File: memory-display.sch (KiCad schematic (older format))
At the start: 1 part, among them J1 TEENSY-LC

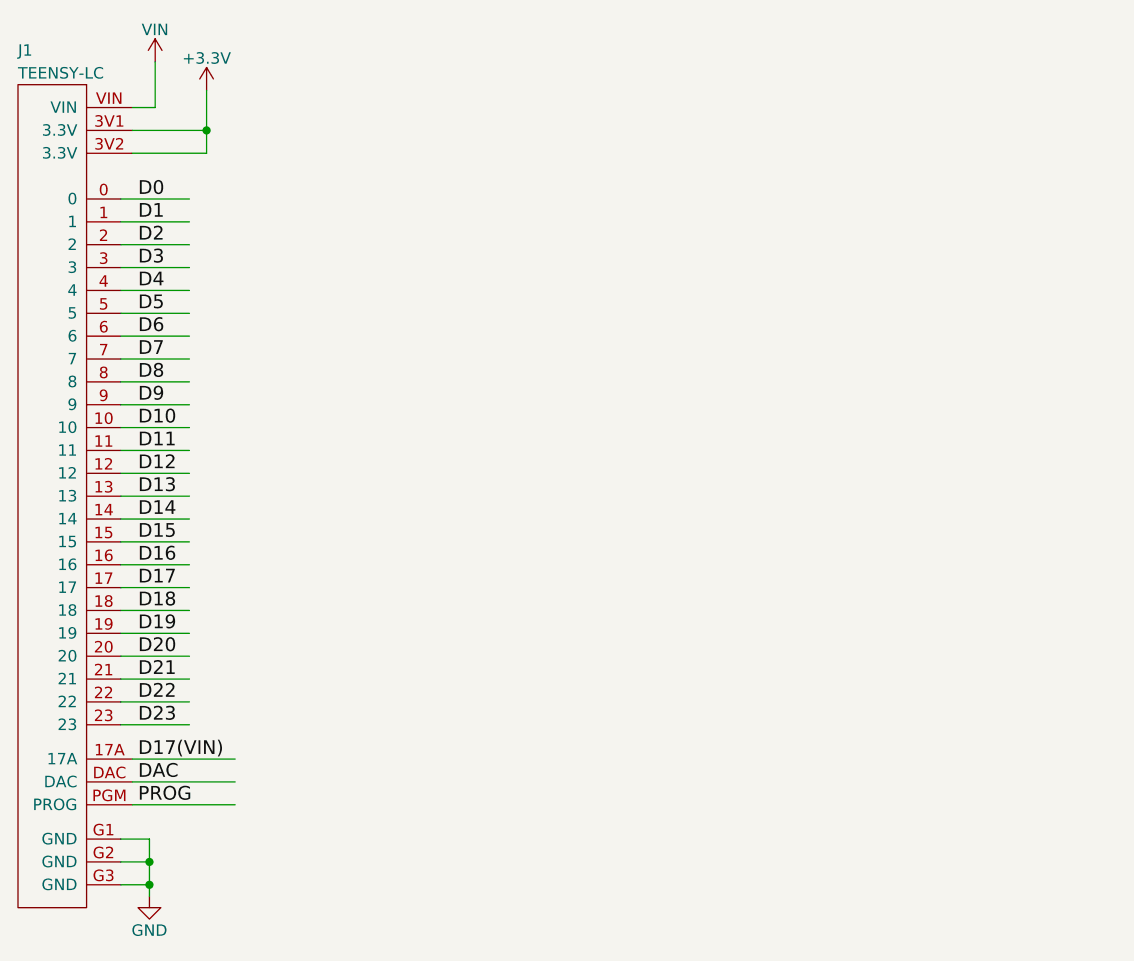
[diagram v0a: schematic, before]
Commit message: finished schematic and start layout
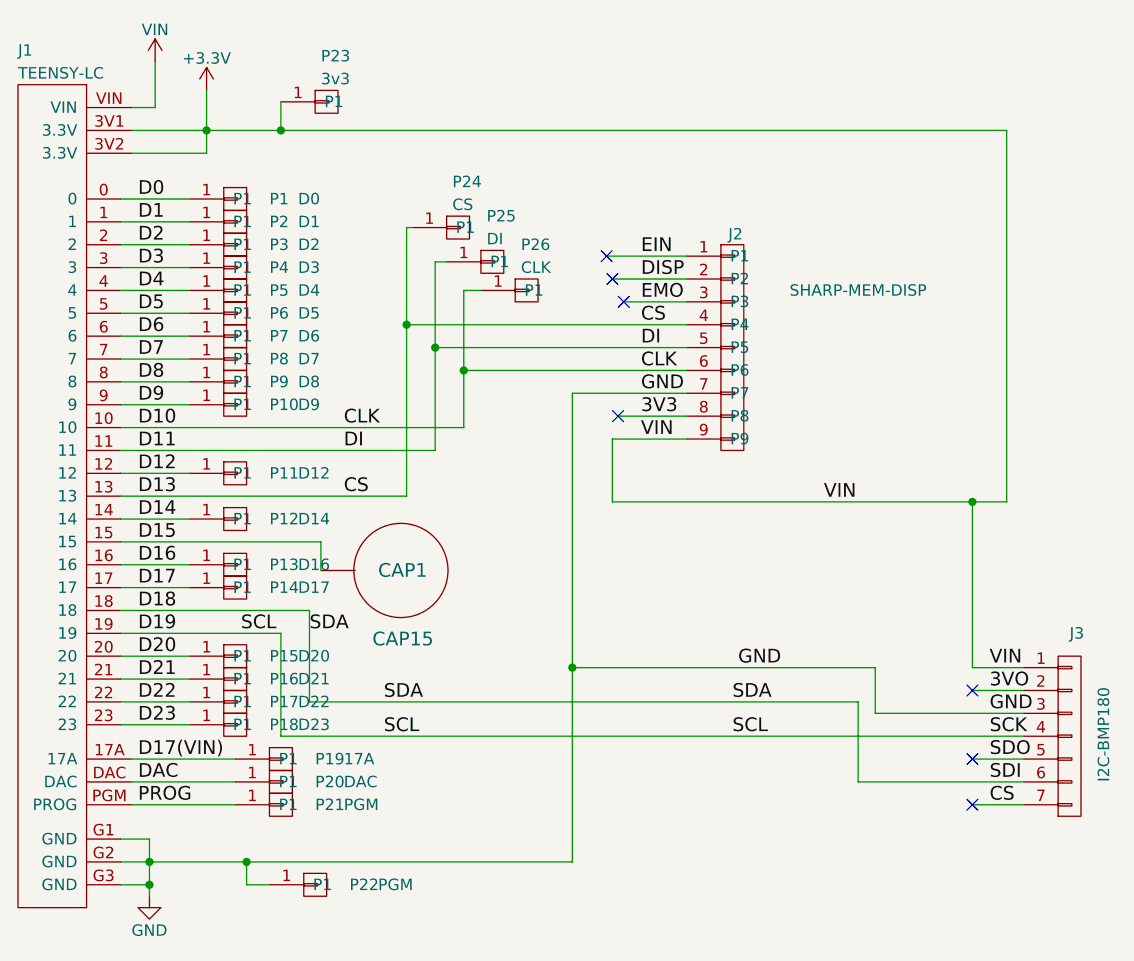
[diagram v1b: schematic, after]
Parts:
- added CAP1: CAP15, Wickerlib:CAPSENSE-CIRCLE-D10MM, symbol CAPSENSE_CIRCLE
- added J2: SHARP-MEM-DISP, Wickerlib:CONN-HEADER-STRAIGHT-P2.54MM-1x09, symbol HEADER-MALE-9POS-TH-1x09-P0.1IN
- added J3: I2C-BMP180, Wickerlib:CONN-HEADER-STRAIGHT-P2.54MM-1x07, symbol HEADER-MALE-7POS-TH-1x07-P0.1IN
- added P1: D0, Wickerlib:CONN-HEADER-STRAIGHT-P2.54MM-1x01, symbol HEADER-MALE-1POS-TH-1x01
- added P10: D9, Wickerlib:CONN-HEADER-STRAIGHT-P2.54MM-1x01, symbol HEADER-MALE-1POS-TH-1x01
- added P11: D12, Wickerlib:CONN-HEADER-STRAIGHT-P2.54MM-1x01, symbol HEADER-MALE-1POS-TH-1x01
- added P12: D14, Wickerlib:CONN-HEADER-STRAIGHT-P2.54MM-1x01, symbol HEADER-MALE-1POS-TH-1x01
- added P13: D16, Wickerlib:CONN-HEADER-STRAIGHT-P2.54MM-1x01, symbol HEADER-MALE-1POS-TH-1x01
- added P14: D17, Wickerlib:CONN-HEADER-STRAIGHT-P2.54MM-1x01, symbol HEADER-MALE-1POS-TH-1x01
- added P15: D20, Wickerlib:CONN-HEADER-STRAIGHT-P2.54MM-1x01, symbol HEADER-MALE-1POS-TH-1x01
- added P16: D21, Wickerlib:CONN-HEADER-STRAIGHT-P2.54MM-1x01, symbol HEADER-MALE-1POS-TH-1x01
- added P17: D22, Wickerlib:CONN-HEADER-STRAIGHT-P2.54MM-1x01, symbol HEADER-MALE-1POS-TH-1x01
- added P18: D23, Wickerlib:CONN-HEADER-STRAIGHT-P2.54MM-1x01, symbol HEADER-MALE-1POS-TH-1x01
- added P19: 17A, Wickerlib:CONN-HEADER-STRAIGHT-P2.54MM-1x01, symbol HEADER-MALE-1POS-TH-1x01
- added P2: D1, Wickerlib:CONN-HEADER-STRAIGHT-P2.54MM-1x01, symbol HEADER-MALE-1POS-TH-1x01
- added P20: DAC, Wickerlib:CONN-HEADER-STRAIGHT-P2.54MM-1x01, symbol HEADER-MALE-1POS-TH-1x01
- added P21, P22: PGM, Wickerlib:CONN-HEADER-STRAIGHT-P2.54MM-1x01, symbol HEADER-MALE-1POS-TH-1x01
- added P23: 3v3, Wickerlib:CONN-HEADER-STRAIGHT-P2.54MM-1x01, symbol HEADER-MALE-1POS-TH-1x01
- added P24: CS, Wickerlib:CONN-HEADER-STRAIGHT-P2.54MM-1x01, symbol HEADER-MALE-1POS-TH-1x01
- added P25: DI, Wickerlib:CONN-HEADER-STRAIGHT-P2.54MM-1x01, symbol HEADER-MALE-1POS-TH-1x01
- added P26: CLK, Wickerlib:CONN-HEADER-STRAIGHT-P2.54MM-1x01, symbol HEADER-MALE-1POS-TH-1x01
- added P3: D2, Wickerlib:CONN-HEADER-STRAIGHT-P2.54MM-1x01, symbol HEADER-MALE-1POS-TH-1x01
- added P4: D3, Wickerlib:CONN-HEADER-STRAIGHT-P2.54MM-1x01, symbol HEADER-MALE-1POS-TH-1x01
- added P5: D4, Wickerlib:CONN-HEADER-STRAIGHT-P2.54MM-1x01, symbol HEADER-MALE-1POS-TH-1x01
- added P6: D5, Wickerlib:CONN-HEADER-STRAIGHT-P2.54MM-1x01, symbol HEADER-MALE-1POS-TH-1x01
- added P7: D6, Wickerlib:CONN-HEADER-STRAIGHT-P2.54MM-1x01, symbol HEADER-MALE-1POS-TH-1x01
- added P8: D7, Wickerlib:CONN-HEADER-STRAIGHT-P2.54MM-1x01, symbol HEADER-MALE-1POS-TH-1x01
- added P9: D8, Wickerlib:CONN-HEADER-STRAIGHT-P2.54MM-1x01, symbol HEADER-MALE-1POS-TH-1x01
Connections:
- net labels added: 3V3, 3VO, CLK, CS, DI, DISP, EIN, EMO, SCK, SCL, SDA, SDI, SDO
- wire segments 36 -> 73
- no-connect marks 0 -> 7
